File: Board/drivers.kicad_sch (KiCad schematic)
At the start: 19 parts, among them U10 74LS257, U18 74LS245, U9 74LS257

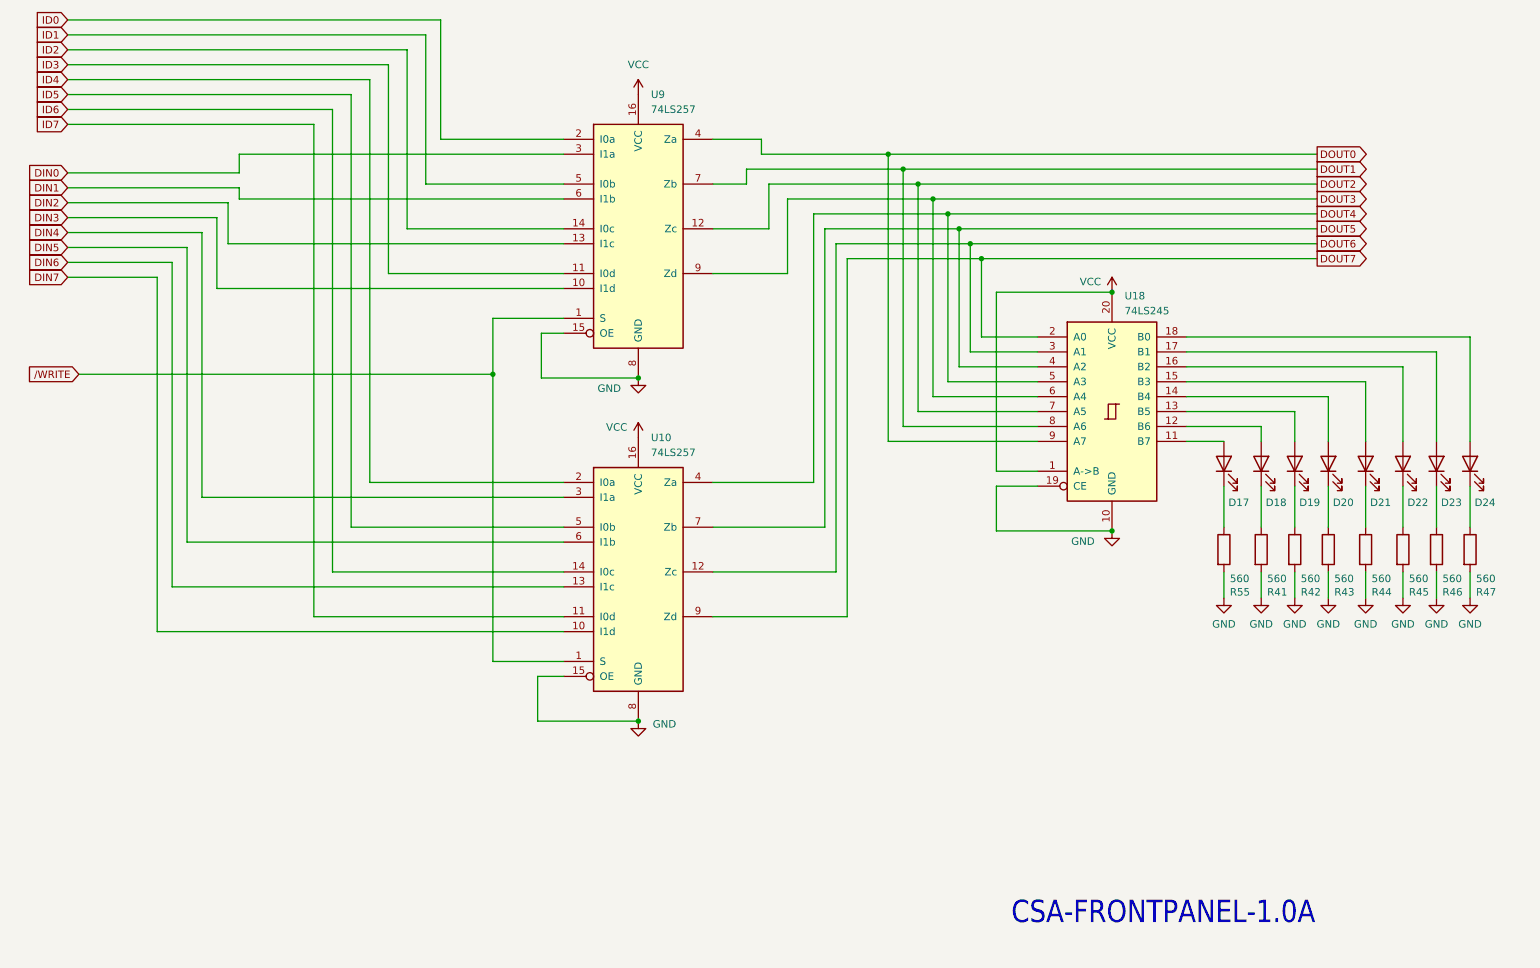
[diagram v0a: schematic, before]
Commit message: More work
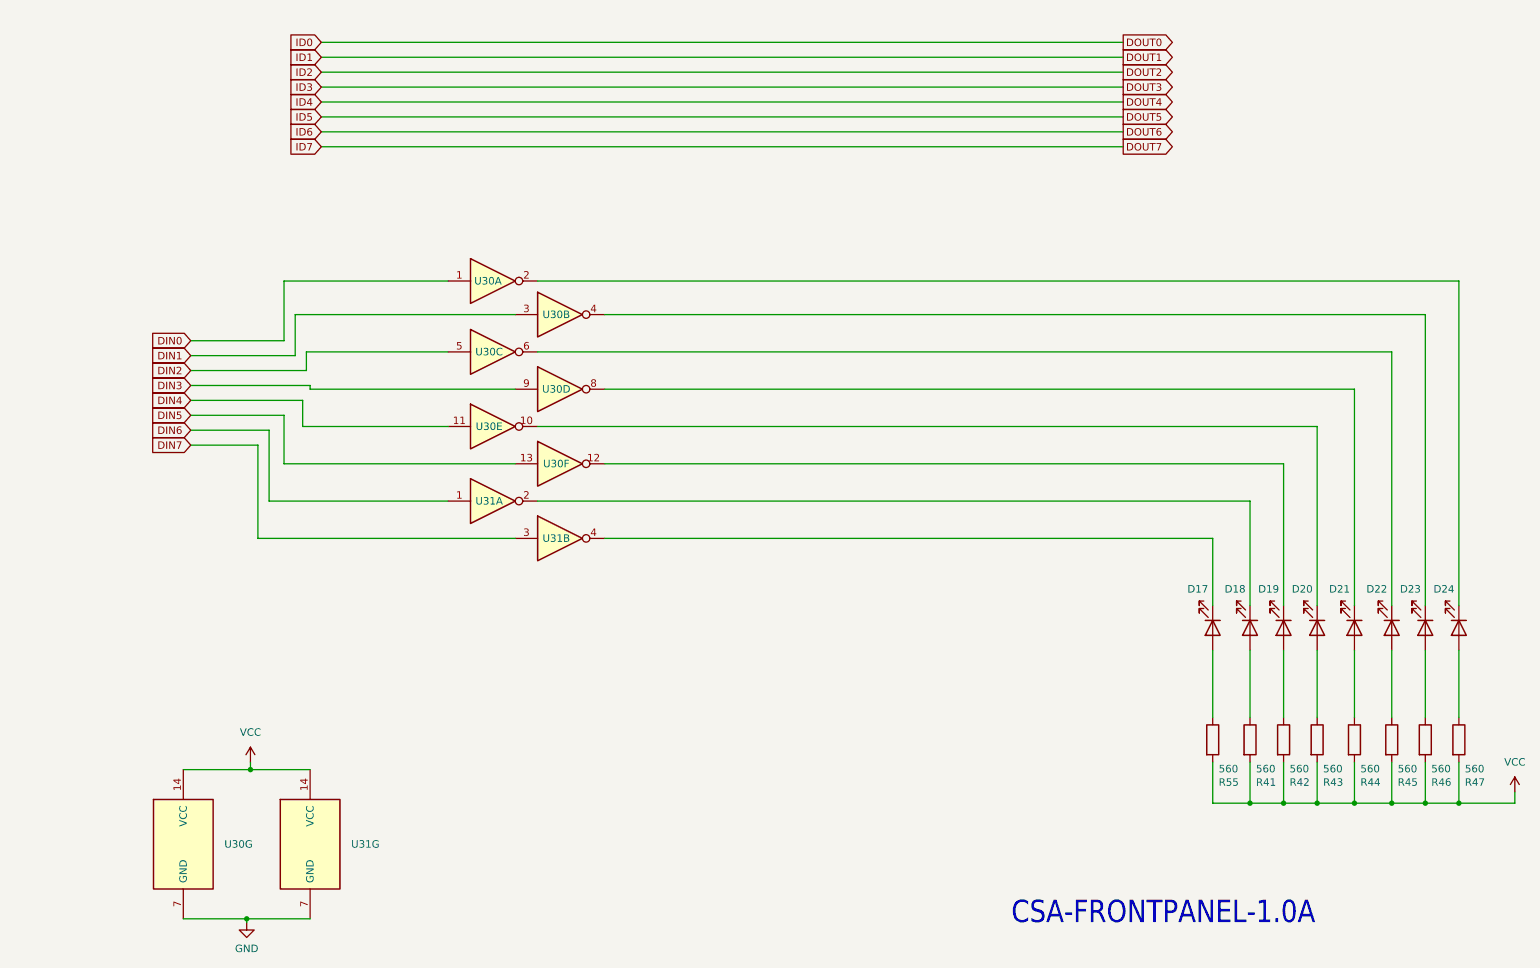
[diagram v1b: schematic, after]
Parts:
- removed U10, U9: 74LS257, Package_SO:SOP-16_4.4x10.4mm_P1.27mm, symbol 74xx:74LS257
- removed U18: 74LS245, Package_SO:TSSOP-20_4.4x5mm_P0.5mm, symbol 74xx:74LS245
- added U30, U31: 74LS06, Package_SO:SOIC-14_3.9x8.7mm_P1.27mm, symbol 74xx:74LS06
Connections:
- net DIN0: now also U30.1
- net DIN1: now also U30.3
- net DIN2: now also U30.5
- net DIN3: now also U30.9
- net DIN4: now also U30.11
- net DIN5: now also U30.13
- net DIN6: now also U31.1
- net DIN7: now also U31.3
- net GND: now also U30.7 (GND), U31.7 (GND); no longer R41.2, R42.2, R43.2, R44.2, R45.2, R46.2, R47.2, R55.2
- net VCC: now also R41.2, R42.2, R43.2, R44.2, R45.2, R46.2, R47.2, R55.2, U30.14 (VCC), U31.14 (VCC)
- net at R42.1: now also D19.2 (A); no longer D19.1 (K)
- net at R55.1: now also D17.2 (A); no longer D17.1 (K)
- net at R47.1: now also D24.2 (A); no longer D24.1 (K)
- net at D18.1 (K): now also U31.2; no longer R41.1
- net at D18.2 (A): now also R41.1
- net at D20.1 (K): now also U30.10; no longer R43.1
- net at D20.2 (A): now also R43.1
- net at R45.1: now also D22.2 (A); no longer D22.1 (K)
- net at D21.1 (K): now also U30.8; no longer R44.1
- net at D21.2 (A): now also R44.1
- net at D23.1 (K): now also U30.4; no longer R46.1
- net at D23.2 (A): now also R46.1
- new net: D19.1 (K), U30.12
- new net: D17.1 (K), U31.4
- new net: D22.1 (K), U30.6
- new net: D24.1 (K), U30.2
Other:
- moved on the sheet: D17, D18, D19, D20, D21, D22, D23, D24, R41, R42, R43, R44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
